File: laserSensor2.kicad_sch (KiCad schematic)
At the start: 7 parts, among them U601 LSM6DSM

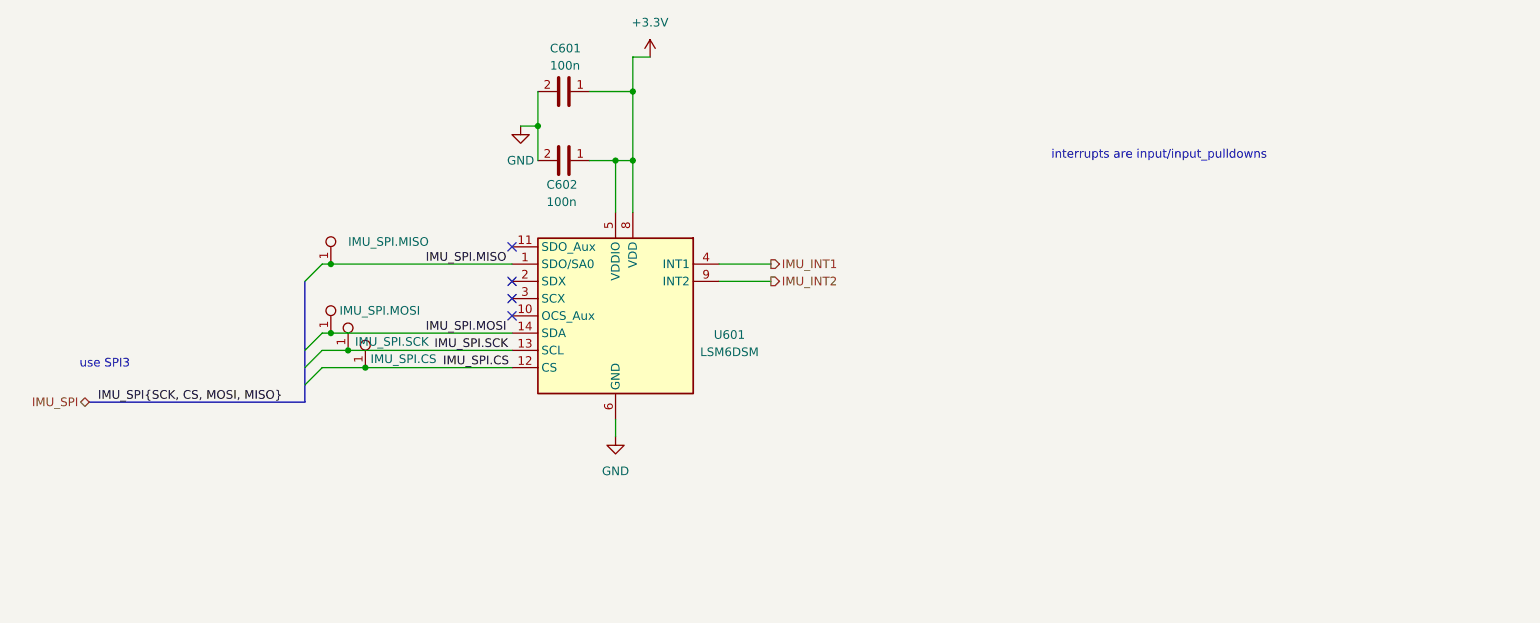
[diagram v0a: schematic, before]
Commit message: preliminary schematic
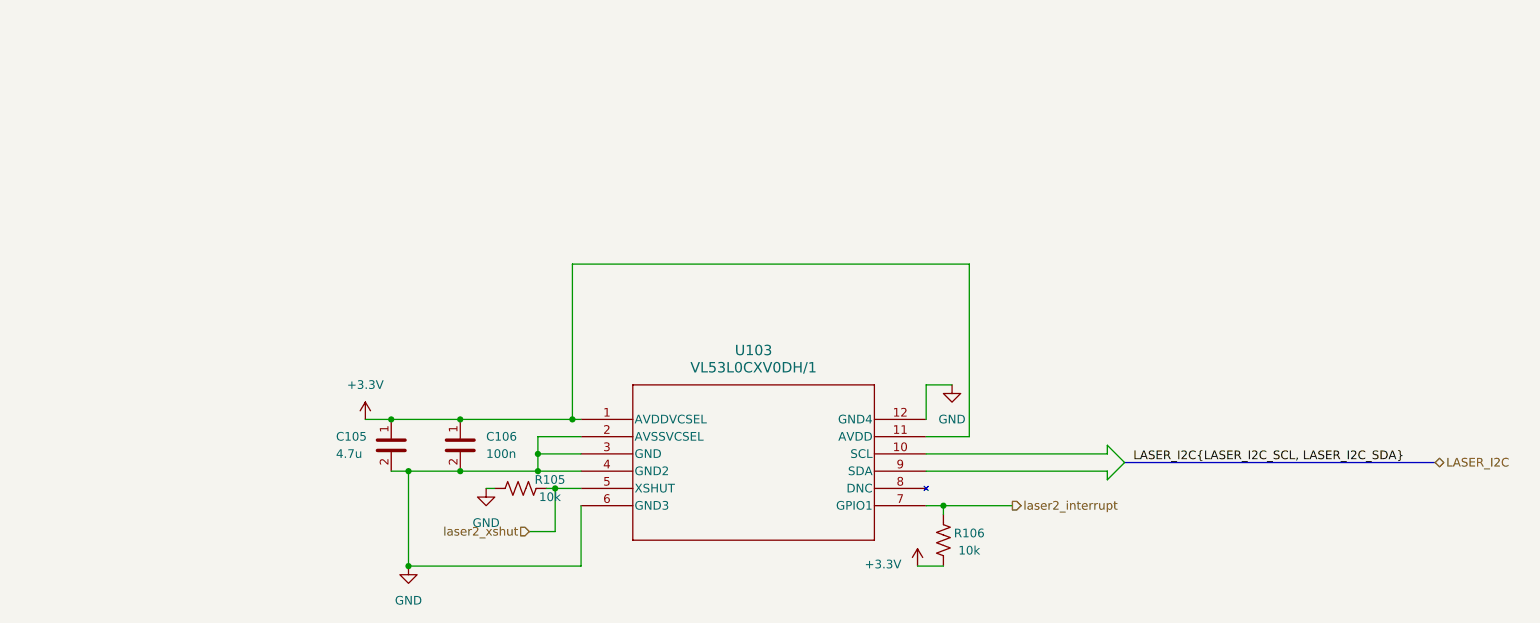
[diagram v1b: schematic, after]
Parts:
- removed C601, C602: 100n, Capacitor_SMD:C_0603_1608Metric_Pad1.08x0.95mm_HandSolder, symbol bfr_capacitors:06035C104KAT2A
- removed TP601: IMU_SPI.MISO, bfr_utilities:TestPoint_Keystone_5019_Miniature, symbol bfr_master:SMD_Test_Point
- removed TP602: IMU_SPI.MOSI, bfr_utilities:TestPoint_Keystone_5019_Miniature, symbol bfr_master:SMD_Test_Point
- removed TP603: IMU_SPI.SCK, bfr_utilities:TestPoint_Keystone_5019_Miniature, symbol bfr_master:SMD_Test_Point
- removed TP604: IMU_SPI.CS, bfr_utilities:TestPoint_Keystone_5019_Miniature, symbol bfr_master:SMD_Test_Point
- removed U601: LSM6DSM, Package_LGA:LGA-14_3x2.5mm_P0.5mm_LayoutBorder3x4y, symbol Sensor_Motion:LSM6DSM
- added C105: 4.7u, Capacitor_SMD:C_0805_2012Metric_Pad1.18x1.45mm_HandSolder, symbol bfr_capacitors:KGM21AR51A475KU
- added C106: 100n, Capacitor_SMD:C_0603_1608Metric_Pad1.08x0.95mm_HandSolder, symbol bfr_capacitors:06035C104KAT2A
- added R105, R106: 10k, Resistor_SMD:R_0603_1608Metric_Pad0.98x0.95mm_HandSolder, symbol bfr_resistors:RMCF0603FT10K0
- added U103: VL53L0CXV0DH/1, LGA12_STM, symbol VL53L0CXV0DH/1:VL53L0CXV0DH_1
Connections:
- net +3.3V: now also C105.1, C106.1, R106.2, U103.1 (AVDDVCSEL), U103.11 (AVDD)
- net GND: now also C105.2, C106.2, R105.1, U103.12 (GND4), U103.2 (AVSSVCSEL), U103.3 (GND), U103.4 (GND2), U103.6 (GND3)
- new net laser2_interrupt: R106.1, U103.7 (GPIO1)
- new net laser2_xshut: R105.2, U103.5 (XSHUT)
- no-connect marks 4 -> 0
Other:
- note removed: "interrupts are input/input_pulldowns"
- note removed: "use SPI3"
